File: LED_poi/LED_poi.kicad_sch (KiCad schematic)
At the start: 43 parts, among them J1 V D G, J10 ICSP, J11 Ext_ACC, J12 RX, J13 TX, J3 V D G, J4 D+, J5 Batt, J6 +5V, J7 KEY, J8 D-, J9 GND, Q1 2N7002, Q2 2N7002, Q3 2N7002, SW1 SW_Push, U1 ATmega32U4-A, U3 ADXL343, U4 TSOP23xx, Y1 16MHz

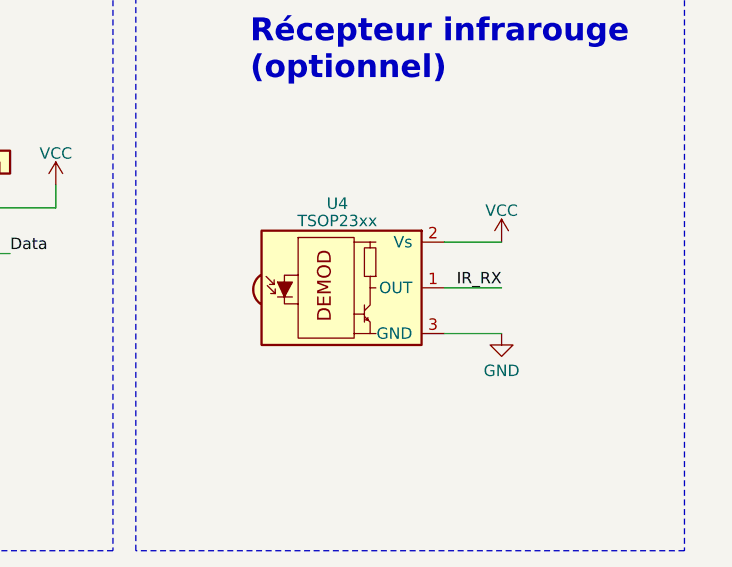
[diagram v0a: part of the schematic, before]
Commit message: a
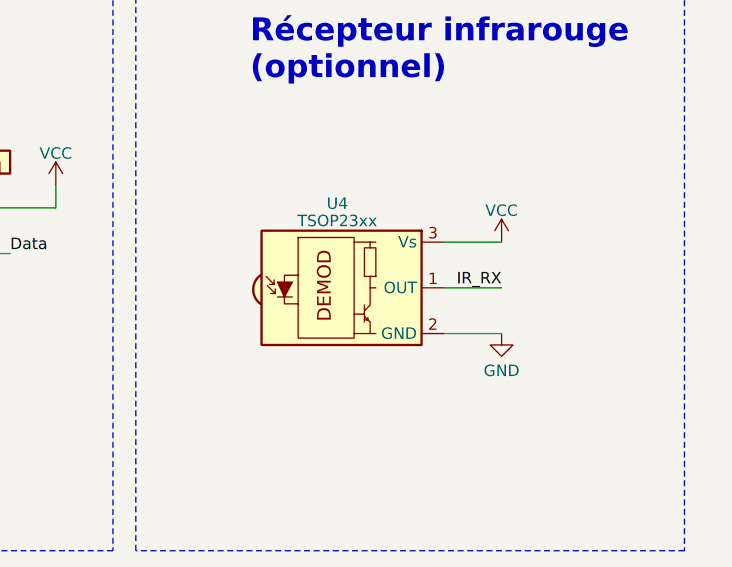
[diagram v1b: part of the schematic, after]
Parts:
- U4: footprint OptoDevice:Vishay_MOLD-3Pin -> OptoDevice:Vishay_MINICAST-3Pin; symbol Interface_Optical:TSOP23xx -> Interface_Optical:TSOP384xx
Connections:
- net GND: now also U4.2 (GND); no longer U4.3 (GND)
- net VCC: now also U4.3 (Vs); no longer U4.2 (Vs)
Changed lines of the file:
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@@
     )
   )
-  (symbol (lib_id "Interface_Optical:TSOP23xx") (at 246.38 48.26 0) (unit 1)
+  (symbol (lib_id "Interface_Optical:TSOP384xx") (at 246.38 48.26 0) (unit 1)
     (in_bom yes) (on_board yes) (dnp no) (fields_autoplaced)
     (property "Reference" "U4" (at 244.645 38.9001 0)
@@
       (effects (font (size 1.27 1.27)))
     )
-    (property "Footprint" "OptoDevice:Vishay_MOLD-3Pin" (at 245.11 57.785 0)
+    (property "Footprint" "OptoDevice:Vishay_MINICAST-3Pin" (at 245.11 57.785 0)
       (effects (font (size 1.27 1.27)) hide)
     )
-    (property "Datasheet" "http://www.vishay.com/docs/82460/tsop45.pdf" (at 262.89 40.64 0)
+    (property "Datasheet" "http://www.vishay.com/docs/82491/tsop382.pdf" (at 262.89 40.64 0)
       (effects (font (size 1.27 1.27)) hide)
     )
